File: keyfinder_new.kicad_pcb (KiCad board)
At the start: 2 copper layers, 38.5 x 27.5 mm, 27 parts, among them J3 Conn_ARM_SWD_TagConnect_TC2030, SW1 SW_Push, SW2 SW_Omron_B3FS, U1 NRF52832, X1 32MHz, X2 32.768kHz

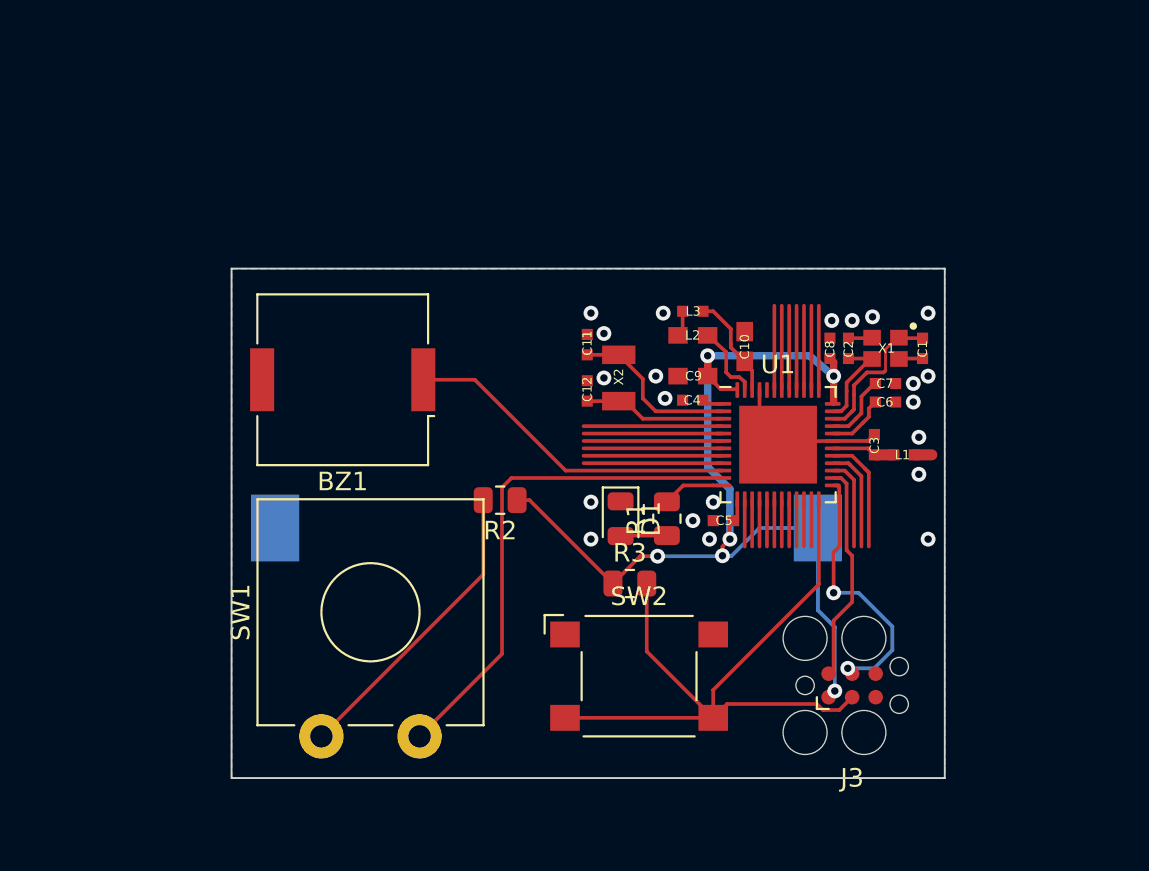
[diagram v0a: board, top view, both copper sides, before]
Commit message: Passage sur le vrai PCB
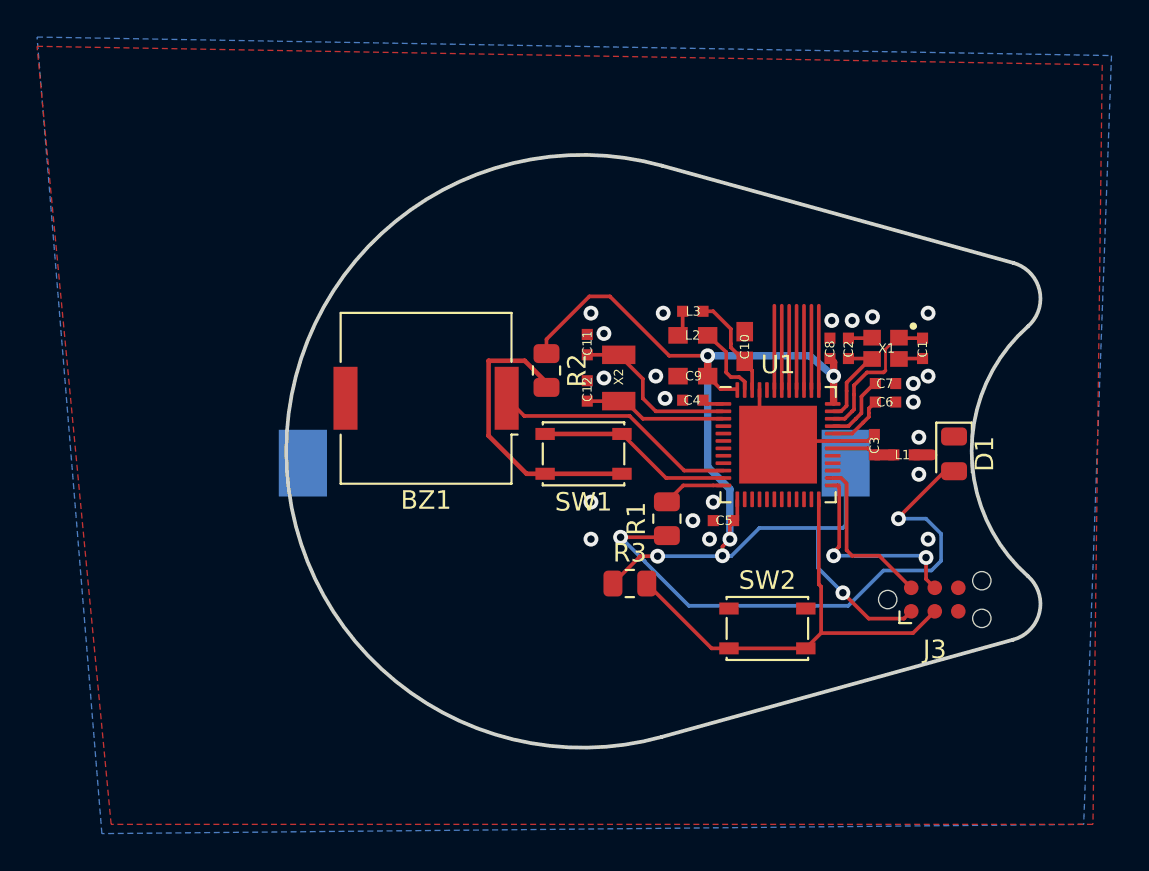
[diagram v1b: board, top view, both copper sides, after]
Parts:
- J3: footprint Connector:Tag-Connect_TC2030-IDC-FP_2x03_P1.27mm_Vertical -> Connector:Tag-Connect_TC2030-IDC-NL_2x03_P1.27mm_Vertical
- R1: value 75 -> 330
- SW1: footprint Button_Switch_THT:SW_CW_GPTS203211B -> Button_Switch_SMD:SW_SPST_PTS810
- SW2: footprint Button_Switch_SMD:SW_SPST_Omron_B3FS-100xP -> Button_Switch_SMD:SW_SPST_PTS810
- moved SW1 20.8 mm to (139.0, 106.5), turned to 180 degrees
- moved D1 18.3 mm to (159.0, 106.5)
- moved R2 7.43 mm to (137.0, 102.0), turned to -90 degrees
- moved SW2 7.39 mm to (148.9, 115.9)
- moved J3 6.43 mm to (158.0, 114.4)
- moved BZ1 4.61 mm to (130.5, 103.5)
- moved BT1 3.81 mm to (138.5, 107.0)
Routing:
- net Net-(D1-A): track 2.51 -> 30.1 mm, vias 0 -> 2
- net /P0.09: track 27.4 -> 10.6 mm
- net /P0.21/RESET: track 39.1 -> 25.0 mm
- net VCC: track 55.7 -> 64.2 mm
- net /P0.07: track 7.50 -> 0.00 mm
- net /P0.06: track 7.50 -> 0.00 mm
- net /P0.05: track 7.50 -> 0.00 mm
- net /P0.04: track 7.50 -> 0.00 mm
- net /P0.03: track 7.50 -> 0.00 mm
- net /P0.02: track 7.50 -> 0.00 mm
- net /P0.24: track 6.27 -> 0.00 mm
- net /P0.23: track 5.59 -> 0.00 mm
- net /P0.22: track 4.91 -> 0.00 mm
- net /P0.08: track 18.2 -> 13.3 mm
- net /SWDCLK: track 14.6 -> 11.1 mm
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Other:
- board size 38.5 x 27.5 mm -> 40.7 x 32 mm
